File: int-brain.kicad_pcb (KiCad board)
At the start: 2 copper layers, 152.4 x 66.5 mm, 105 parts, among them J1 PWR, J10 Left, J11 Right, J12 1MA_ENC, J13 1MB_ENC, J14 2MA_ENC, J15 2MB_ENC, J16 USB_A, J2 UART0, J3 I2C0, J4 PWR, J5 1MA, J6 1MB, J7 2MA, J8 2MB, J9 MPU9250, SW1 SW_Push, U1 L298N, U2 ESP32-DevKitC, U3 L298N, U4 TPS5430DDA, U7 PCA9635, U8 TPS5430DDA

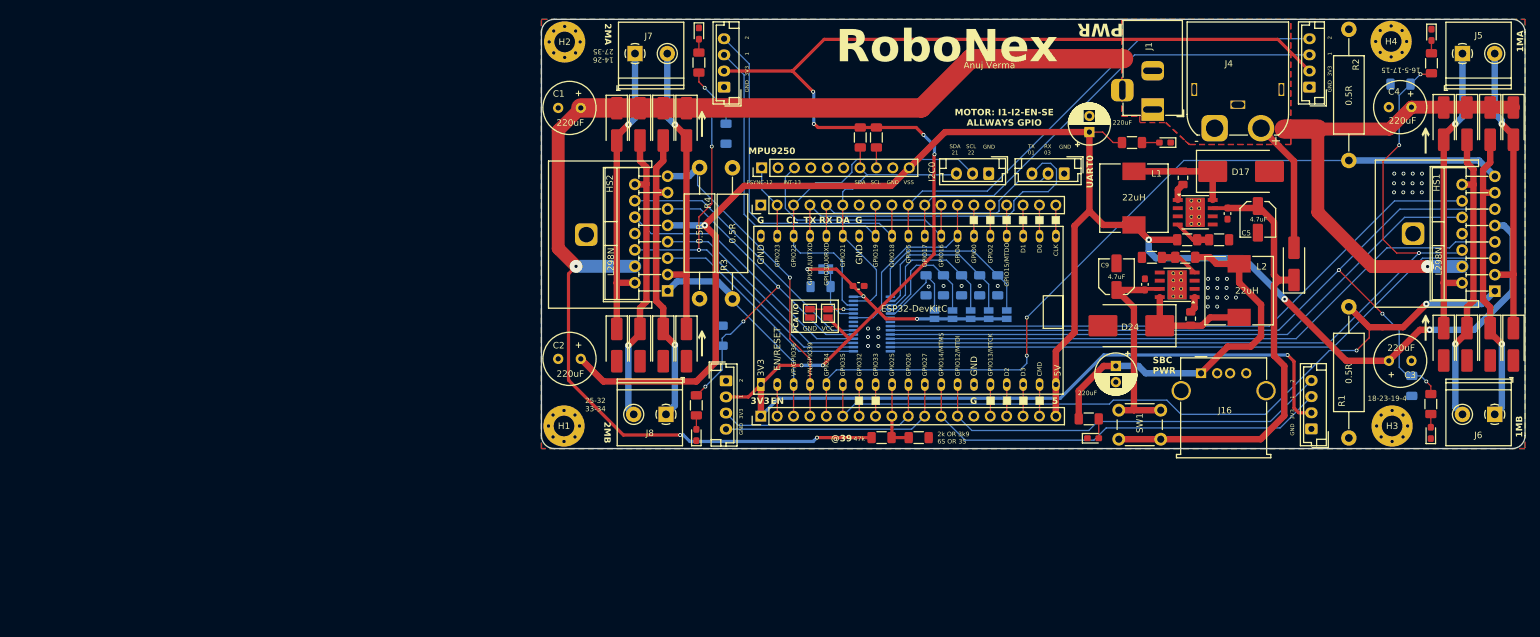
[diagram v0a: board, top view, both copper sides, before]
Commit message: placed?
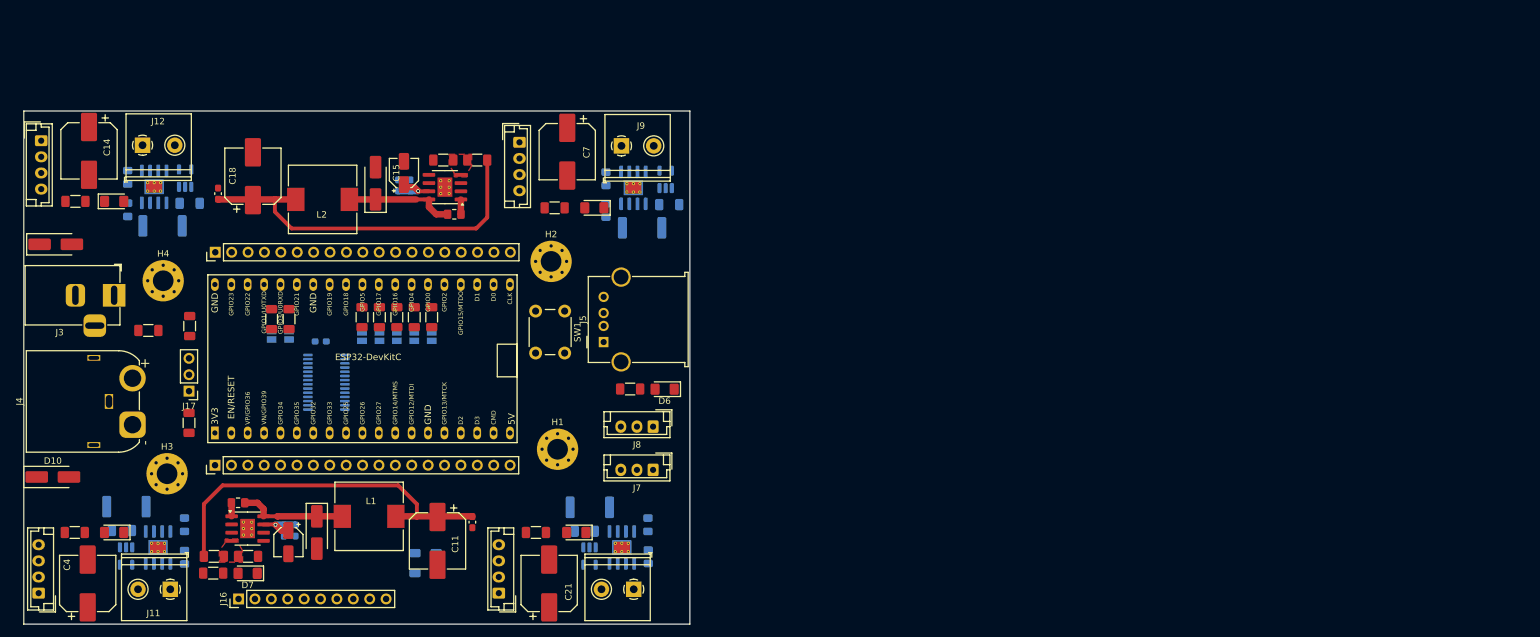
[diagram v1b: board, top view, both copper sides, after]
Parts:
- removed D11, D12, D13, D14, D15, D16, D23: D, Diode_SMD:D_SMA_Handsoldering
- removed D17, D24: B340, Diode_SMD:D_SMC_Handsoldering
- removed D18, D19, D20, D21: LED, LED_SMD:LED_0603_1608Metric_Pad1.05x0.95mm_HandSolder
- removed D22, D25: PWR, LED_SMD:LED_0603_1608Metric_Pad1.05x0.95mm_HandSolder
- removed HS1, HS2: Heatsink_Pad, heatsink:Heatsink_PI48
- removed JP0: A0, Jumper:SolderJumper-2_P1.3mm_Open_Pad1.0x1.5mm
- added C14: 220uF, Capacitor_SMD:CP_Elec_8x10.5, F.Cu at (47.8, 73.9)
- added C15: 4.7uF, Capacitor_SMD:CP_Elec_4x5.4, F.Cu at (96.6, 77.3)
- added C16: 4.7uF, Capacitor_SMD:C_0603_1608Metric_Pad1.08x0.95mm_HandSolder, B.Cu at (95.7, 79.2)
- added C17: 10nF, Capacitor_SMD:C_0805_2012Metric_Pad1.18x1.45mm_HandSolder, F.Cu at (104.4, 83.7)
- added C18: 330uF, Capacitor_SMD:CP_Elec_8x10.5, F.Cu at (73.2, 77.8)
- added C19: 10nF, Capacitor_SMD:C_0805_2012Metric_Pad1.18x1.45mm_HandSolder, B.Cu at (134.4, 131.8)
- added C20: 1uF, Capacitor_SMD:C_0805_2012Metric_Pad1.18x1.45mm_HandSolder, B.Cu at (134.4, 136.8)
- added C21: 220uF, Capacitor_SMD:CP_Elec_8x10.5, F.Cu at (119.1, 140.9)
- added C22: 10nF, Capacitor_SMD:C_0603_1608Metric_Pad1.08x0.95mm_HandSolder, B.Cu at (78.0, 132.7)
- added C23: 10nF, Capacitor_SMD:C_0603_1608Metric_Pad1.08x0.95mm_HandSolder, B.Cu at (97.6, 79.2)
- added C24: 10nF, Capacitor_SMD:C_0603_1608Metric_Pad1.08x0.95mm_HandSolder, F.Cu at (107.2, 131.4)
- added C25: 10nF, Capacitor_SMD:C_0603_1608Metric_Pad1.08x0.95mm_HandSolder, F.Cu at (67.8, 80.5)
- added J17: Conn_01x03, Connector_PinHeader_2.54mm:PinHeader_1x03_P2.54mm_Vertical, F.Cu at (63.3, 111.1)
- added R29: 10k, Resistor_SMD:R_1206_3216Metric_Pad1.30x1.75mm_HandSolder, F.Cu at (78.8, 100.0)
- added R30: 3k9, Resistor_SMD:R_1206_3216Metric_Pad1.30x1.75mm_HandSolder, F.Cu at (63.3, 116.0)
- added U10: ~, Package_SO:SOIC-8-1EP_3.9x4.9mm_P1.27mm_EP2.29x3mm_ThermalVias, F.Cu at (103.0, 79.5)
- added U11: DRV8251ADDAR, Package_SO:SOIC-8-1EP_3.9x4.9mm_P1.27mm_EP2.29x3mm_ThermalVias, B.Cu at (130.4, 135.3)
- added U12: INA139, Package_TO_SOT_SMD:SOT-23-5_HandSoldering, B.Cu at (125.3, 136.7)
- added U5: DRV8251ADDAR, Package_SO:SOIC-8-1EP_3.9x4.9mm_P1.27mm_EP2.29x3mm_ThermalVias, B.Cu at (132.2, 79.6)
- added U6: INA139, Package_TO_SOT_SMD:SOT-23-5_HandSoldering, B.Cu at (137.2, 78.3)
- added U9: INA139, Package_TO_SOT_SMD:SOT-23-5_HandSoldering, B.Cu at (62.7, 78.1)
- C1: value 220uF -> 100nF; footprint Capacitor_THT:C_Radial_D8.0mm_H11.5mm_P3.50mm -> Capacitor_SMD:C_0603_1608Metric_Pad1.08x0.95mm_HandSolder; moved to B.Cu
- C10: value 4.7uF -> 10nF; footprint Capacitor_SMD:C_0603_1608Metric_Pad1.08x0.95mm_HandSolder -> Capacitor_SMD:C_0805_2012Metric_Pad1.18x1.45mm_HandSolder
- C11: value 10nF -> 330uF; footprint Capacitor_SMD:C_0805_2012Metric_Pad1.18x1.45mm_HandSolder -> Capacitor_SMD:CP_Elec_8x10.5
- C12: value 220uF -> 10nF; footprint Capacitor_THT:CP_Radial_D6.3mm_P2.50mm -> Capacitor_SMD:C_0805_2012Metric_Pad1.18x1.45mm_HandSolder; moved to B.Cu
- C13: value 100nF -> 1uF; footprint Capacitor_SMD:C_0603_1608Metric_Pad1.08x0.95mm_HandSolder -> Capacitor_SMD:C_0805_2012Metric_Pad1.18x1.45mm_HandSolder; moved to B.Cu
- C2: value 220uF -> 10nF; footprint Capacitor_THT:C_Radial_D8.0mm_H11.5mm_P3.50mm -> Capacitor_SMD:C_0805_2012Metric_Pad1.18x1.45mm_HandSolder; moved to B.Cu
- C3: value 220uF -> 1uF; footprint Capacitor_THT:C_Radial_D8.0mm_H11.5mm_P3.50mm -> Capacitor_SMD:C_0805_2012Metric_Pad1.18x1.45mm_HandSolder; moved to B.Cu
- C4: footprint Capacitor_THT:C_Radial_D8.0mm_H11.5mm_P3.50mm -> Capacitor_SMD:CP_Elec_8x10.5
- C5: value 4.7uF -> 10nF; footprint Capacitor_SMD:C_Elec_5x5.8 -> Capacitor_SMD:C_0805_2012Metric_Pad1.18x1.45mm_HandSolder; moved to B.Cu
- C6: value 4.7uF -> 1uF; footprint Capacitor_SMD:C_0603_1608Metric_Pad1.08x0.95mm_HandSolder -> Capacitor_SMD:C_0805_2012Metric_Pad1.18x1.45mm_HandSolder; moved to B.Cu
- C7: value 10nF -> 220uF; footprint Capacitor_SMD:C_0805_2012Metric_Pad1.18x1.45mm_HandSolder -> Capacitor_SMD:CP_Elec_8x10.5
- C8: value 220uF -> 4.7uF; footprint Capacitor_THT:CP_Radial_D6.3mm_P2.50mm -> Capacitor_SMD:CP_Elec_4x5.4
- C9: footprint Capacitor_SMD:C_Elec_5x5.8 -> Capacitor_SMD:C_0603_1608Metric_Pad1.08x0.95mm_HandSolder; moved to B.Cu
- D1, D2, D3, D4: value D -> LED; footprint Diode_SMD:D_SMA_Handsoldering -> LED_SMD:LED_1206_3216Metric_Pad1.42x1.75mm_HandSolder
- D6, D7: value D -> PWR; footprint Diode_SMD:D_SMA_Handsoldering -> LED_SMD:LED_1206_3216Metric_Pad1.42x1.75mm_HandSolder
- D8, D9: value D -> SS54
- J1: value PWR -> Right; footprint Connector_BarrelJack:BarrelJack_Horizontal -> Connector_PinHeader_2.54mm:PinHeader_1x19_P2.54mm_Vertical
- J10: value Left -> 2MB; footprint Connector_PinHeader_2.54mm:PinHeader_1x19_P2.54mm_Vertical -> TerminalBlock_Philmore:TerminalBlock_Philmore_TB132_1x02_P5.00mm_Horizontal
- J11: value Right -> 1MB; footprint Connector_PinHeader_2.54mm:PinHeader_1x19_P2.54mm_Vertical -> TerminalBlock_Philmore:TerminalBlock_Philmore_TB132_1x02_P5.00mm_Horizontal
- J12: value 1MA_ENC -> 1MA; footprint Connector_JST:JST_EH_B4B-EH-A_1x04_P2.50mm_Vertical -> TerminalBlock_Philmore:TerminalBlock_Philmore_TB132_1x02_P5.00mm_Horizontal
- J13: value 1MB_ENC -> 1MA_ENC
- J14: value 2MA_ENC -> 1MB_ENC
- J15: value 2MB_ENC -> 2MA_ENC
- J16: value USB_A -> MPU9250; footprint Connector_USB:USB_A_Molex_67643_Horizontal -> Connector_PinHeader_2.54mm:PinHeader_1x10_P2.54mm_Vertical
- J2: value UART0 -> Left; footprint Connector_JST:JST_EH_B3B-EH-A_1x03_P2.50mm_Vertical -> Connector_PinHeader_2.54mm:PinHeader_1x19_P2.54mm_Vertical
- J3: value I2C0 -> PWR; footprint Connector_JST:JST_EH_B3B-EH-A_1x03_P2.50mm_Vertical -> Connector_BarrelJack:BarrelJack_Horizontal
- J5: value 1MA -> USB_A; footprint TerminalBlock_Philmore:TerminalBlock_Philmore_TB132_1x02_P5.00mm_Horizontal -> Connector_USB:USB_A_Molex_67643_Horizontal
- J6: value 1MB -> 2MB_ENC; footprint TerminalBlock_Philmore:TerminalBlock_Philmore_TB132_1x02_P5.00mm_Horizontal -> Connector_JST:JST_EH_B4B-EH-A_1x04_P2.50mm_Vertical
- J7: value 2MA -> I2C0; footprint TerminalBlock_Philmore:TerminalBlock_Philmore_TB132_1x02_P5.00mm_Horizontal -> Connector_JST:JST_EH_B3B-EH-A_1x03_P2.50mm_Vertical
- J8: value 2MB -> UART0; footprint TerminalBlock_Philmore:TerminalBlock_Philmore_TB132_1x02_P5.00mm_Horizontal -> Connector_JST:JST_EH_B3B-EH-A_1x03_P2.50mm_Vertical
- J9: value MPU9250 -> 2MA; footprint Connector_PinHeader_2.54mm:PinHeader_1x10_P2.54mm_Vertical -> TerminalBlock_Philmore:TerminalBlock_Philmore_TB132_1x02_P5.00mm_Horizontal
- JP1: value A1 -> A0
- JP2: value A2 -> A1
- JP3: value A3 -> A2
- JP4: value A4 -> A3
- JP5: value A5 -> A4
- JP6: value VCC -> A5; moved to B.Cu
- JP7: value GND -> VCC; moved to B.Cu
- R1, R2, R3: value 0.5R -> 220R; footprint Resistor_THT:R_Axial_DIN0414_L11.9mm_D4.5mm_P20.32mm_Horizontal -> Resistor_SMD:R_1206_3216Metric_Pad1.30x1.75mm_HandSolder
- R10: value 47k -> 3k9
- R12, R21: moved to F.Cu
- R13, R14: value 10k -> 470R; moved to F.Cu
- R15: value 10k -> 4.7k
- R16: moved to B.Cu
- R17: value 4.7k -> 10mR; footprint Resistor_SMD:R_1206_3216Metric_Pad1.30x1.75mm_HandSolder -> Resistor_SMD:R_2512_6332Metric_Pad1.40x3.35mm_HandSolder; moved to B.Cu
- R18, R20, R28: value 10k -> 24k
- R19: value 10k -> 10mR; footprint Resistor_SMD:R_1206_3216Metric_Pad1.30x1.75mm_HandSolder -> Resistor_SMD:R_2512_6332Metric_Pad1.40x3.35mm_HandSolder
- R22: value 10k -> 3.16k; moved to F.Cu
- R23: value 470R -> 10mR; footprint Resistor_SMD:R_1206_3216Metric_Pad1.30x1.75mm_HandSolder -> Resistor_SMD:R_2512_6332Metric_Pad1.40x3.35mm_HandSolder; moved to B.Cu
- R24: value 10k -> 24k; moved to B.Cu
- R25: value 3.24k -> 10k
- R26: value 10k -> 3.16k
- R27: value 3.24k -> 10mR; footprint Resistor_SMD:R_1206_3216Metric_Pad1.30x1.75mm_HandSolder -> Resistor_SMD:R_2512_6332Metric_Pad1.40x3.35mm_HandSolder; moved to B.Cu
- R4: value 0.5R -> 10k; footprint Resistor_THT:R_Axial_DIN0414_L11.9mm_D4.5mm_P20.32mm_Horizontal -> Resistor_SMD:R_1206_3216Metric_Pad1.30x1.75mm_HandSolder
- R6, R7: value 220R -> 10k
- R8: value 220R -> 47k
- R9: value 470R -> 10k
- U1: value L298N -> PCA9635; footprint Package_TO_SOT_THT:TO-220-15_P2.54x2.54mm_StaggerOdd_Lead4.58mm_Vertical -> Package_SO:TSSOP-28_4.4x9.7mm_P0.65mm; moved to B.Cu
- U2: footprint PCM_Espressif:ESP32-DevKitC -> PCM_Espressif:ESP32-DevKitC-slim
- U3: value L298N -> DRV8251ADDAR; footprint Package_TO_SOT_THT:TO-220-15_P2.54x2.54mm_StaggerOdd_Lead4.58mm_Vertical -> Package_SO:SOIC-8-1EP_3.9x4.9mm_P1.27mm_EP2.29x3mm_ThermalVias; moved to B.Cu
- U4: value TPS5430DDA -> INA139; footprint Package_SO:TI_SO-PowerPAD-8_ThermalVias -> Package_TO_SOT_SMD:SOT-23-5_HandSoldering; moved to B.Cu
- U7: value PCA9635 -> ~; footprint Package_SO:TSSOP-28_4.4x9.7mm_P0.65mm -> Package_SO:SOIC-8-1EP_3.9x4.9mm_P1.27mm_EP2.29x3mm_ThermalVias; moved to F.Cu
- U8: value TPS5430DDA -> DRV8251ADDAR; footprint Package_SO:TI_SO-PowerPAD-8_ThermalVias -> Package_SO:SOIC-8-1EP_3.9x4.9mm_P1.27mm_EP2.29x3mm_ThermalVias; moved to B.Cu
- moved J6 227.3 mm to (40.0, 142.4), turned to 90 degrees
- moved D5 223.0 mm to (42.6, 88.3), turned to 0 degrees
- moved C4 214.7 mm to (47.6, 140.9), turned to 90 degrees
- moved D2 208.1 mm to (51.7, 133.0), turned to 180 degrees
- moved D1 206.4 mm to (51.7, 81.7), turned to 0 degrees
- moved R2 205.6 mm to (45.6, 133.0), turned to 0 degrees
- moved D7 201.4 mm to (72.4, 139.3), turned to 180 degrees
- moved R1 198.0 mm to (45.7, 81.7), turned to 180 degrees
- moved H4 193.8 mm to (59.3, 94.0)
- moved C3 192.5 mm to (62.6, 136.8), turned to 90 degrees
- moved H3 189.9 mm to (59.9, 123.9)
- moved R14 188.0 mm to (67.0, 139.3), turned to 0 degrees
- moved U1 181.6 mm to (84.6, 109.7), turned to 180 degrees
- moved D8 180.6 mm to (83.1, 133.0)
- moved R12 178.6 mm to (76.1, 100.0), turned to -90 degrees
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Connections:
- C1 pad 1: GND -> +3.3V
- C1 pad 2: VS -> GND
- C10 pad 1: /buck2/BUCK_VIN -> Net-(U7-BOOT)
- C10 pad 2: GND -> /buck1/BUCK_OUT
- C11 pad 1: Net-(U8-BOOT) -> VSS
- C11 pad 2: /buck2/BUCK_OUT -> GND
- C12 pad 1: /buck2/VOUT -> +3.3V
- C13 pad 1: +3.3V -> VS
- C2 pad 1: GND -> +3.3V
- C2 pad 2: VSS -> GND
- C3 pad 1: GND -> VS
- C3 pad 2: VSS -> GND
- C4 pad 1: GND -> VS
- C4 pad 2: VS -> GND
- C5 pad 1: BUCK_VS -> +3.3V
- C6 pad 1: BUCK_VS -> VS
- C7 pad 1: Net-(U4-BOOT) -> VS
- C7 pad 2: /buck1/BUCK_OUT -> GND
- C8 pad 1: VSS -> VS
- C9 pad 1: /buck2/BUCK_VIN -> VS
- D1 pad 1: VS -> GND
- D1 pad 2: /1MA1 -> /1MAL
- D10 pad 1: /2MA1 -> VS
- D10 pad 2: GND -> /VS_UNSAFE
- D2 pad 1: /1MA1 -> GND
- D2 pad 2: GND -> /1MBL
- D3 pad 1: VS -> GND
- D3 pad 2: /1MA2 -> /2MAL
- D4 pad 1: /1MA2 -> GND
- D4 pad 2: GND -> /2MBL
- D5 pad 2: /1MB1 -> /VS_UNSAFE
- D6 pad 1: /1MB1 -> GND
- D6 pad 2: GND -> /PWR_LED_2
- D7 pad 1: VS -> GND
- D7 pad 2: /1MB2 -> /PWR_LED_1
- D8 pad 1: /1MB2 -> /buck1/BUCK_OUT
- D9 pad 1: VS -> /buck2/BUCK_OUT
- D9 pad 2: /2MA1 -> GND
- J1 pad 1: VS -> GND
- J1 pad 2: GND -> FSYNC
- J1 pad 3: (no net) -> SCL0
- J10 pad 1: +3.3V -> /2MB1
- J10 pad 2: /EN -> /2MB2
- J11 pad 1: GND -> /1MB1
- J11 pad 2: FSYNC -> /1MB2
- J12 pad 1: GND -> /1MA1
- J12 pad 2: +3.3V -> /1MA2
- J13 pad 3: /1MA1_ENC -> /2MA1_ENC
- J13 pad 4: /1MA2_ENC -> /2MA2_ENC
- J14 pad 3: /2MB1_ENC -> /1MA1_ENC
- J14 pad 4: /2MB2_ENC -> /1MA2_ENC
- J15 pad 3: /1MB1_ENC -> /2MB1_ENC
- J15 pad 4: /1MB2_ENC -> /2MB2_ENC
- J16 pad 1: /buck2/VOUT -> FSYNC
- J16 pad 3: unconnected-(J16-D+-Pad3) -> INT
- J16 pad 4: GND -> unconnected-(J16-Pin_4-Pad4)
- J16 pad 5: GND -> unconnected-(J16-Pin_5-Pad5)
- J2 pad 1: GND -> +3.3V
- J2 pad 2: /RX0 -> /EN
- J2 pad 3: /TX0 -> 2MB_SENSE
- J3 pad 1: GND -> /VS_UNSAFE
- J3 pad 2: SCL0 -> GND
- J3 pad 3: SDA0 -> GND
- J4 pad 2: VS -> /VS_UNSAFE
- J5 pad 1: /1MA1 -> /buck2/VOUT
- J5 pad 2: /1MA2 -> unconnected-(J5-D--Pad2)
- J6 pad 1: /1MB1 -> GND
- J6 pad 2: /1MB2 -> +3.3V
- J7 pad 1: /2MA1 -> GND
- J7 pad 2: /2MA2 -> SCL0
- J8 pad 1: /2MB1 -> GND
- J8 pad 2: /2MB2 -> /RX0
- J9 pad 1: FSYNC -> /2MA1
- J9 pad 2: unconnected-(J9-Pin_2-Pad2) -> /2MA2
- JP1 pad 2: /PCA_A1 -> /PCA_A0
- JP2 pad 2: /PCA_A2 -> /PCA_A1
- JP3 pad 2: /PCA_A3 -> /PCA_A2
- JP4 pad 2: /PCA_A4 -> /PCA_A3
- JP5 pad 2: /PCA_A5 -> /PCA_A4
- JP6 pad 2: /PCA_IO -> /PCA_A5
- JP7 pad 1: GND -> +3.3V
- R1 pad 1: 1MA_SENSE -> /1MA_EN
- R1 pad 2: GND -> /1MAL
- R10 pad 1: VS -> /3S
- R10 pad 2: VBATT -> GND
- R11 pad 1: VBATT -> GND
- R11 pad 2: GND -> /PCA_A4
- R12 pad 1: /1MA_EN -> GND
- R12 pad 2: GND -> /PCA_A5
- R13 pad 1: /2MA_EN -> /buck2/VOUT
- R13 pad 2: GND -> /PWR_LED_2
- R14 pad 1: /1MB_EN -> VSS
- R14 pad 2: GND -> /PWR_LED_1
- R15 pad 1: /2MB_EN -> SCL0
- R15 pad 2: GND -> +3.3V
- R16 pad 1: SCL0 -> SDA0
- R17 pad 1: SDA0 -> /motor-driver-2/IPROPI
- R17 pad 2: +3.3V -> GND
- R18 pad 1: GND -> 1MB_SENSE
- R18 pad 2: /PCA_A1 -> GND
- R19 pad 1: GND -> /motor-driver-3/IPROPI
- R19 pad 2: /PCA_A2 -> GND
- R2 pad 1: 1MB_SENSE -> /1MB_EN
- R2 pad 2: GND -> /1MBL
- R20 pad 1: GND -> 2MA_SENSE
- R20 pad 2: /PCA_A3 -> GND
- R21 pad 1: GND -> VSS
- R21 pad 2: /PCA_A4 -> /buck1/BUCK_VSENSE
- R22 pad 1: GND -> /buck1/BUCK_VSENSE
- R22 pad 2: /PCA_A5 -> GND
- R23 pad 1: /buck2/VOUT -> /motor-driver-1/IPROPI
- R23 pad 2: /PWR_LED_2 -> GND
- R24 pad 1: VSS -> 1MA_SENSE
- R24 pad 2: /buck1/BUCK_VSENSE -> GND
- R25 pad 1: /buck1/BUCK_VSENSE -> /buck2/VOUT
- R25 pad 2: GND -> /buck2/BUCK_VSENSE
- R26 pad 1: /buck2/VOUT -> /buck2/BUCK_VSENSE
- R26 pad 2: /buck2/BUCK_VSENSE -> GND
- R27 pad 1: /buck2/BUCK_VSENSE -> /motor-driver-4/IPROPI
- R28 pad 1: GND -> 2MB_SENSE
- R28 pad 2: /PCA_A0 -> GND
- R3 pad 1: 2MB_SENSE -> /2MA_EN
- R3 pad 2: GND -> /2MAL
- R4 pad 1: 2MA_SENSE -> GND
- R4 pad 2: GND -> /PCA_A0
- R5 pad 1: /1MA_EN -> /2MB_EN
- R5 pad 2: /1MAL -> /2MBL
- R6 pad 1: /1MB_EN -> GND
- R6 pad 2: /1MBL -> /PCA_A1
- R7 pad 1: /2MA_EN -> GND
- R7 pad 2: /2MAL -> /PCA_A2
- R8 pad 1: /2MB_EN -> VS
- R8 pad 2: /2MBL -> VBATT
- R9 pad 1: VSS -> GND
- R9 pad 2: /PWR_LED_1 -> /PCA_A3
- U1 pad 1: 1MA_SENSE -> /PCA_A0
- U1 pad 10: /1MB1_IN -> /2MA_IN1
- U1 pad 11: /1MB_EN -> /2MA_IN2
- U1 pad 12: /1MB2_IN -> /2MB_IN1
- U1 pad 13: /1MB1 -> /2MB_IN2
- U1 pad 14: /1MB2 -> GND
- U1 pad 15: 1MB_SENSE -> /1MB_IN1
- U1 pad 2: /1MA1 -> /PCA_A1
- U1 pad 3: /1MA2 -> /PCA_A2
- U1 pad 4: VS -> /PCA_A3
- U1 pad 5: /1MA1_IN -> /PCA_A4
- U1 pad 6: /1MA_EN -> /2MA_EN
- U1 pad 7: /1MA2_IN -> /2MB_EN
- U1 pad 8: GND -> unconnected-(U1-LED2-Pad8)
- U1 pad 9: VSS -> unconnected-(U1-LED3-Pad9)
- U3 pad 1: 2MB_SENSE -> /motor-driver-2/IPROPI
- U3 pad 2: /2MA1 -> /1MB_IN2
- U3 pad 3: /2MA2 -> /1MB_IN1
- U3 pad 4: VS -> +3.3V
- U3 pad 5: /2MA1_IN -> VS
- U3 pad 6: /2MA_EN -> /1MB1
- U3 pad 7: /2MA2_IN -> GND
- U3 pad 8: GND -> /1MB2
- U3 pad 9: VSS -> GND
- U4 pad 1: Net-(U4-BOOT) -> 1MB_SENSE
- U4 pad 2: unconnected-(U4-NC-Pad2) -> GND
- U4 pad 3: unconnected-(U4-NC-Pad3) -> /motor-driver-2/IPROPI
- U4 pad 4: /buck1/BUCK_VSENSE -> GND
- U4 pad 5: unconnected-(U4-EN-Pad5) -> +3.3V
- U7 pad 1: /PCA_A0 -> Net-(U7-BOOT)
- U7 pad 2: /PCA_A1 -> unconnected-(U7-NC-Pad2)
- U7 pad 3: /PCA_A2 -> unconnected-(U7-NC-Pad3)
- U7 pad 4: /PCA_A3 -> /buck1/BUCK_VSENSE
- U7 pad 5: /PCA_A4 -> unconnected-(U7-ENA-Pad5)
- U7 pad 6: unconnected-(U7-LED0-Pad6) -> GND
- U7 pad 7: unconnected-(U7-LED1-Pad7) -> VS
- U7 pad 8: /1MB2_IN -> /buck1/BUCK_OUT
- U7 pad 9: /1MB_EN -> GND
- U8 pad 1: Net-(U8-BOOT) -> /motor-driver-1/IPROPI
- U8 pad 2: unconnected-(U8-NC-Pad2) -> /1MA_IN2
- U8 pad 3: unconnected-(U8-NC-Pad3) -> /1MA_IN1
- U8 pad 4: /buck2/BUCK_VSENSE -> +3.3V
- U8 pad 5: unconnected-(U8-EN-Pad5) -> VS
- U8 pad 6: GND -> /1MA1
- U8 pad 7: /buck2/BUCK_VIN -> GND
- U8 pad 8: /buck2/BUCK_OUT -> /1MA2
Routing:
- net +3.3V: track 327.3 -> 0.00 mm, vias 10 -> 0
- net VS: track 289.0 -> 7.35 mm, vias 4 -> 1
- net VSS: track 266.0 -> 57.3 mm, vias 4 -> 0
- net /1MA_EN: track 130.7 -> 0.00 mm, vias 3 -> 0
- net 1MB_SENSE: track 128.5 -> 0.00 mm, vias 2 -> 0
- net /1MB_EN: track 127.7 -> 0.00 mm, vias 3 -> 0
- net 1MA_SENSE: track 121.2 -> 0.00 mm, vias 2 -> 0
- net /1MA2_IN: track 99.9 -> 0.00 mm
- net /1MA1_IN: track 99.4 -> 0.00 mm
- net /1MB2_IN: track 96.6 -> 0.00 mm
- net /1MB1_IN: track 96.1 -> 0.00 mm
- net /1MA2_ENC: track 77.6 -> 0.00 mm
- net /2MA_EN: track 74.1 -> 0.00 mm, vias 3 -> 0
- net /1MA1_ENC: track 74.1 -> 0.00 mm
- net BUCK_VS: track 73.7 -> 0.00 mm
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- added copper zone on F.Cu, net /buck1/BUCK_VSENSE
- added copper zone on F.Cu, net /buck2/BUCK_VSENSE
- removed copper zone on B.Cu, net GND
- removed copper zone on F.Cu, net GND
- removed copper zone on F.Cu, net VS
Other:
- board size 152.4 x 66.5 mm -> 103.2 x 79.5 mm
- board text removed: "+"
- board text removed: "1"
- board text removed: "14-26 27-35"
- board text removed: "16-5-17-15"
- board text removed: "18-23-19-4"
- board text removed: "2"
- board text removed: "25-32 33-34"
- board text removed: "2k OR 3k9 6S OR 3S"
- board text removed: "3V3"
- board text removed: "47k"
- board text removed: "5"
- board text removed: "@39"
- board text removed: "Anuj Verma"
- board text removed: "CL"
- board text removed: "DA"
- board text removed: "EN"
- board text removed: "FSYNC-12"
- board text removed: "G"
- board text removed: "GND"
- board text removed: "INT-13"
- board text removed: "MOTOR: I1-I2-EN-SE ALLWAYS GPIO"
- board text removed: "PCA I/O"
- board text removed: "RX"
- board text removed: "RX 03"
- board text removed: "RoboNex"
- board text removed: "SBC PWR"
- board text removed: "SCL"
- board text removed: "SCL 22"
- board text removed: "SDA"
- board text removed: "SDA 21"
- board text removed: "TX"
- board text removed: "TX 01"
- board text removed: "VSS"
- board text removed: "→"
